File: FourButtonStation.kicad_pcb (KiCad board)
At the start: 2 copper layers, 106 x 63.5 mm, 50 parts, among them J1 AC IN, J10 AC IN, J2 External 3V, J3 TTL, J4 TODO: AVOX Adapter might need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, J5 Conn_WallSocket, J6 USB_B_Micro, J7 Conn_WallSocket, J8 Conn_WallSocket, J9 Conn_WallSocket, K1 G5LE-1, K2 G5LE-1, K3 G5LE-1, K4 G5LE-1, Q1 MMBT3904, Q3 MMBT3904, SW1 POWER, SW2 RST, U1 CH340C, U10 SM4007PL, U11 D882_C9634, U2 radio-receiver, U3 ESP-07, U4 SM4007PL, U5 D882_C9634, U6 SM4007PL, U7 D882_C9634, U8 SM4007PL, U9 D882_C9634

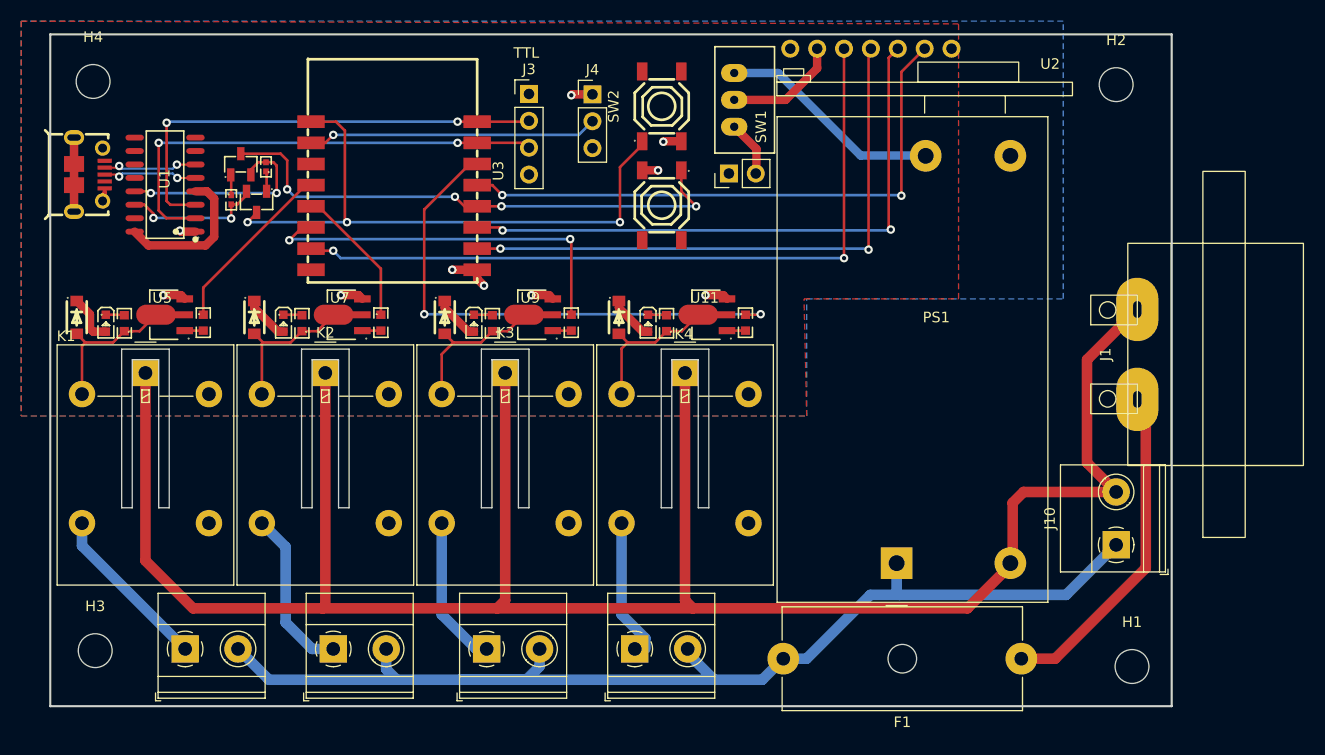
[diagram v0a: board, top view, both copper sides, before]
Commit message: Prepare for production
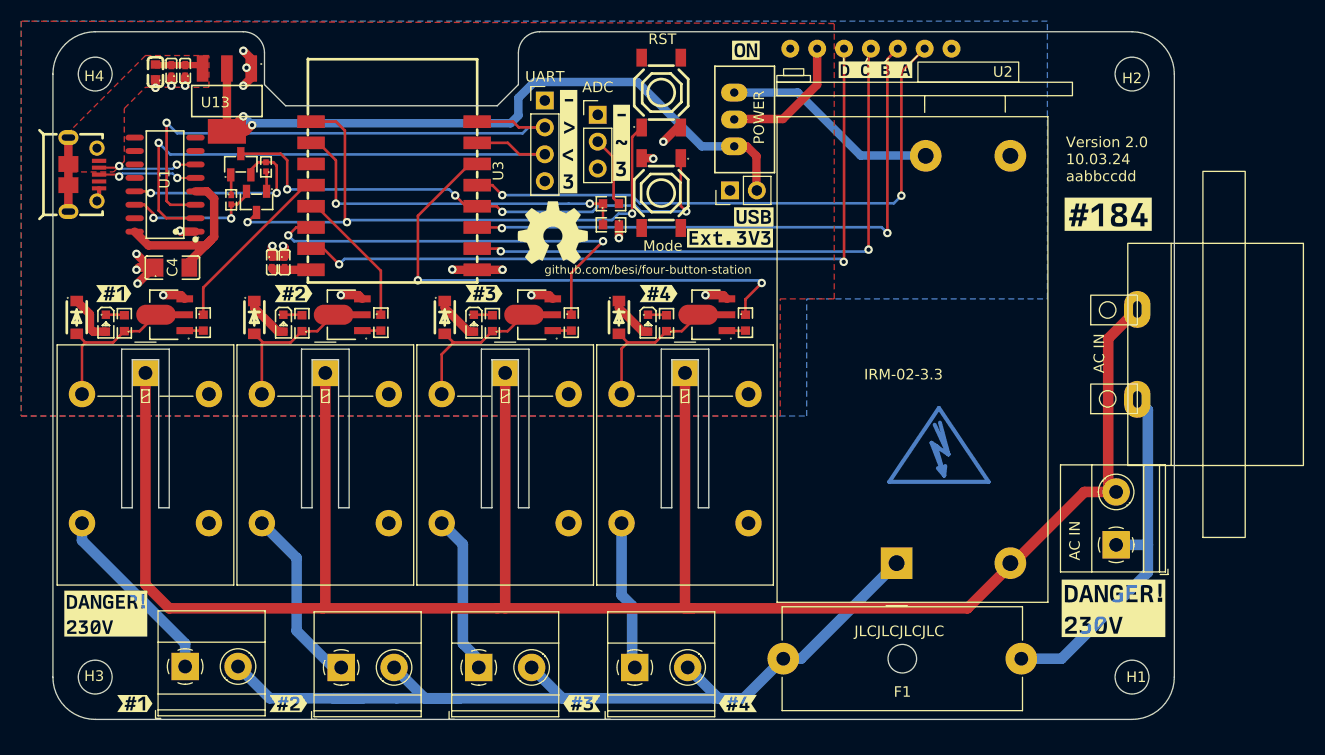
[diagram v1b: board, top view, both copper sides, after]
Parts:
- removed SWe: Mode, jlc_footprints:SW-SMD_4P-L5.1-W5.1-P3.70-LS6.5-TL-2
- added C1: 10u, jlc_footprints:C0402, F.Cu at (29.8, 93.5)
- added C2: 100n, jlc_footprints:C0402, F.Cu at (28.4, 93.5)
- added C3: 22u, jlc_footprints:C0603, F.Cu at (26.9, 93.5)
- added C4: 100u, jlc_footprints:C1206, F.Cu at (28.6, 112.0)
- added C5: 100n, jlc_footprints:C0402, F.Cu at (39.1, 111.5)
- added C6: 10u, jlc_footprints:C0402, F.Cu at (38.0, 111.5)
- added R11: 22k, jlc_footprints:R0603, F.Cu at (70.0, 106.0)
- added R12: 10k, jlc_footprints:R0603, F.Cu at (70.0, 108.0)
- added SW5: Mode, jlc_footprints:SW-SMD_4P-L5.1-W5.1-P3.70-LS6.5-TL-2, F.Cu at (74.8, 105.0)
- added SYM1: SYM_Flash_XLarge, Symbol:Symbol_HighVoltage_Type2_CopperTop_VerySmall, B.Cu at (101.0, 129.5)
- added Sym2: github.com/besi/four-button-station, Symbol:OSHW-Symbol_6.7x6mm_SilkScreen, F.Cu at (64.5, 108.8)
- added U13: AMS1117-3_3, jlc_footprints:SOT-223-3_L6.5-W3.4-P2.30-LS7.0-BR, F.Cu at (33.7, 96.2)
- added kibuzzard-65EDF79E: G***, kibuzzard-65EDF79E, F.Cu at (117.0, 107.0)
- added kibuzzard-65EDF7BF: G***, kibuzzard-65EDF7BF, F.Cu at (95.0, 93.3)
- added kibuzzard-65EE2541: G***, kibuzzard-65EE2541, F.Cu at (58.0, 114.5)
- added kibuzzard-65EE2549: G***, kibuzzard-65EE2549, F.Cu at (39.5, 153.2)
- added kibuzzard-65EE2549: G***, kibuzzard-65EE2549, F.Cu at (40.0, 114.5)
- added kibuzzard-65EE2550: G***, kibuzzard-65EE2550, F.Cu at (25.0, 153.2)
- added kibuzzard-65EE2550: G***, kibuzzard-65EE2550, F.Cu at (23.0, 114.5)
- added kibuzzard-65EE2558: G***, kibuzzard-65EE2558, F.Cu at (74.5, 114.5)
- added kibuzzard-65EE261E: G***, kibuzzard-65EE261E, F.Cu at (82.8, 91.5)
- added kibuzzard-65EE2681: G***, kibuzzard-65EE2681, F.Cu at (81.2, 109.2)
- added kibuzzard-65EE2746: G***, kibuzzard-65EE2746, F.Cu at (66.0, 100.1)
- added kibuzzard-65EE278E: G***, kibuzzard-65EE278E, F.Cu at (117.5, 144.2)
- added kibuzzard-65EE27C8: G***, kibuzzard-65EE27C8, F.Cu at (82.0, 153.2)
- added kibuzzard-65EE27E0: G***, kibuzzard-65EE27E0, F.Cu at (67.2, 153.2)
- added kibuzzard-65EE2811: G***, kibuzzard-65EE2811, F.Cu at (22.2, 144.8)
- added kibuzzard-65EE298C: G***, kibuzzard-65EE298C, F.Cu at (83.5, 107.2)
- added kibuzzard-65EE35B8: G***, kibuzzard-65EE35B8, F.Cu at (71.0, 100.2)
- J3: value TTL -> UART
- J4: value TODO: AVOX Adapter might need voltage divider -> ADC
- moved H3 2.50 mm to (21.2, 150.8)
- moved J4 1.99 mm to (68.8, 97.6)
- moved J7 1.90 mm to (44.5, 149.8)
- moved J8 1.90 mm to (57.5, 149.8)
- moved SW1 1.85 mm to (81.7, 95.5)
- moved H2 1.80 mm to (119.2, 93.8)
- moved J9 1.75 mm to (72.2, 149.8)
- moved J5 1.66 mm to (29.8, 149.8)
- moved J3 1.62 mm to (63.8, 96.2)
- moved J2 1.60 mm to (81.2, 104.8)
- moved SW2 1.30 mm to (74.8, 95.5)
- moved H1 1.00 mm to (119.2, 150.8)
- moved H4 0.73 mm to (21.2, 93.8)
- moved J6 0.53 mm to (20.2, 103.2)
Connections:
- net POWX renamed POW3V3
- J10 pad 1: /Nullleiter -> /AC_FUSE
- J4 pad 2: ADC -> Net-(J4-Pin_2)
- J6 pad 1: VBUS -> +5V
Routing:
- net POW3V3: track 5.31 -> 68.4 mm, vias 0 -> 2
- net /Nullleiter: track 109.4 -> 89.3 mm
- net GND: track 27.8 -> 45.4 mm, vias 10 -> 21
- net TX: track 44.9 -> 54.4 mm, vias 2 -> 1
- net +3V3: track 42.8 -> 51.7 mm
- net RX: track 45.4 -> 54.0 mm, vias 2 -> 1
- net ADC: track 27.4 -> 34.4 mm, vias 1 -> 2
- net Net-(J4-Pin_2): track 0.00 -> 6.69 mm
- net +5V: track 0.00 -> 4.60 mm
- net Relay3: track 36.3 -> 40.6 mm
- net /Phase: track 207.1 -> 203.5 mm
- net /AC_FUSE: track 31.7 -> 35.1 mm
- net /AC1: track 15.9 -> 17.6 mm
- net RESET: track 57.3 -> 58.8 mm
- net /AC4: track 12.8 -> 14.2 mm
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- added copper zone on F.Cu, net +5V
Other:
- board size 106 x 63.5 mm -> 106 x 65 mm
- board text added: "JLCJLCJLCJLC"
- board text added: "Version 2.0 10.03.24 aabbccdd"
